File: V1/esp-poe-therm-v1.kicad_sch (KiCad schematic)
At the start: 46 parts, among them J1 USB_C_Receptacle_USB2.0, J2 RJ45 JACK, Q1 UMH3N, Q2 WPM2015-3/TR, Q3 LMUN2211LT1G, SW1 RESET, U4 CH340C, U5 ESP32-WROOM-32UE-N4, U6 LAN8710A, U7 AHT20

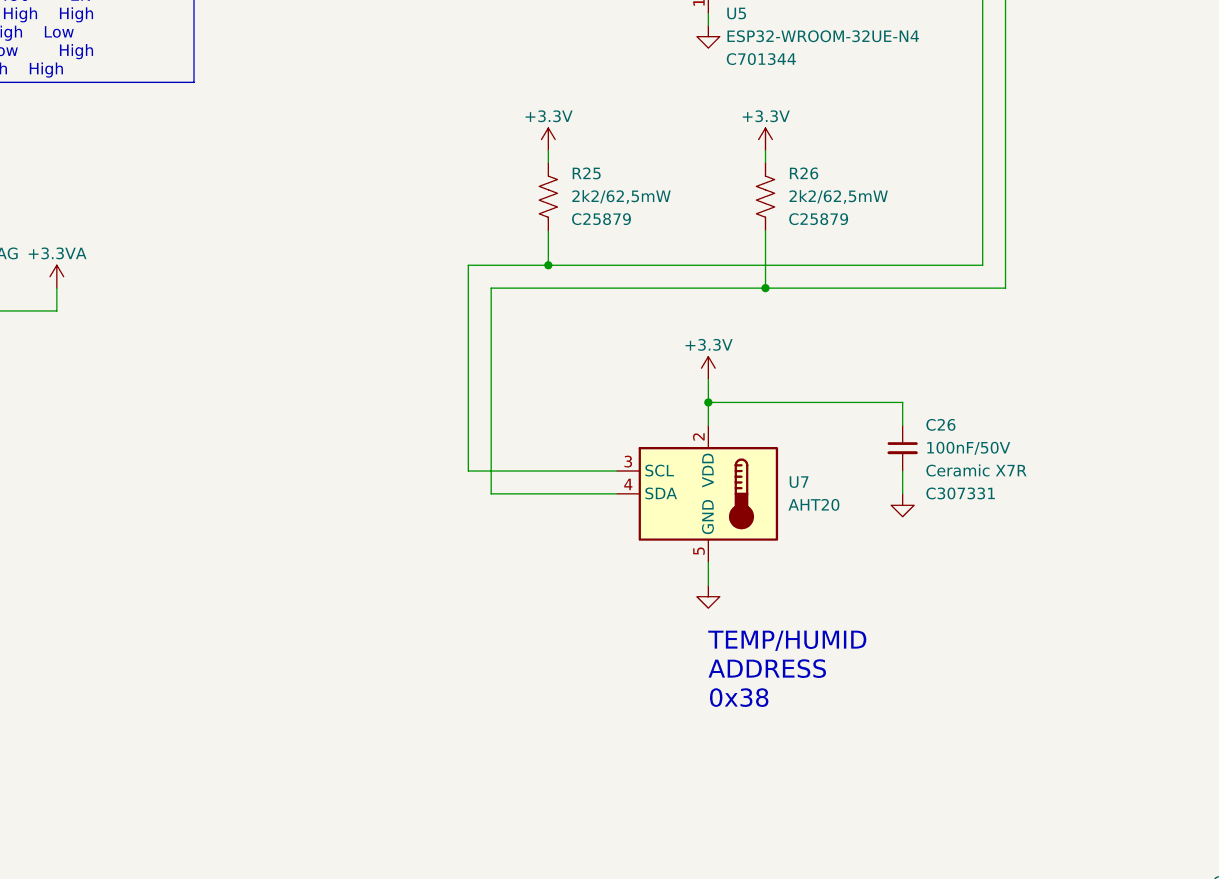
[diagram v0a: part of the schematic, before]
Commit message: dev
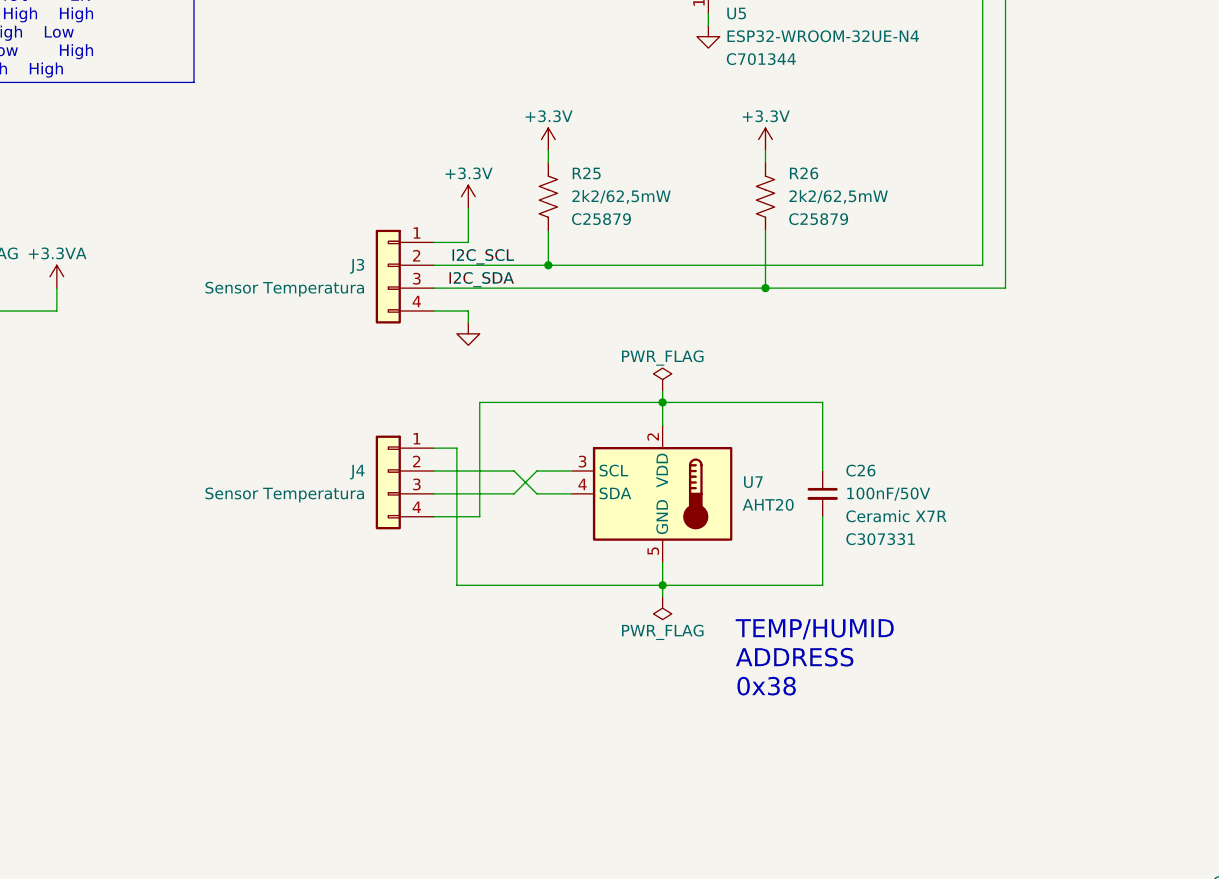
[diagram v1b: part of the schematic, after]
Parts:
- added J3: Sensor Temperatura, Connector_JST:JST_PH_B4B-PH-K_1x04_P2.00mm_Vertical, symbol Connector_Generic:Conn_01x04
- added J4: Sensor Temperatura, Connector_JST:JST_PH_S4B-PH-K_1x04_P2.00mm_Horizontal, symbol Connector_Generic:Conn_01x04
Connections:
- net +3.3V: now also J3.1 (Pin_1); no longer C26.1, U7.2 (VDD)
- net GND: now also J3.4 (Pin_4); no longer C26.2, U7.5 (GND)
- net I2C_SCL: now also J3.2 (Pin_2); no longer U7.3 (SCL)
- net I2C_SDA: now also J3.3 (Pin_3); no longer U7.4 (SDA)
- new net: C26.2, J4.1 (Pin_1), U7.5 (GND)
- new net: J4.2 (Pin_2), U7.4 (SDA)
- new net: J4.3 (Pin_3), U7.3 (SCL)
- new net: C26.1, J4.4 (Pin_4), U7.2 (VDD)
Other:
- moved on the sheet: C26, U7
